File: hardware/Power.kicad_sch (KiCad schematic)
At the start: 33 parts, among them J1 JST XH, J2 JST XH, J22 JST XH, J23 JST XH, J24 JST XH, J25 JST XH, J26 JST XH, J27 JST XH, Q1 NCE40P40K, U4 AMS1117-3.3, U5 DCBuck

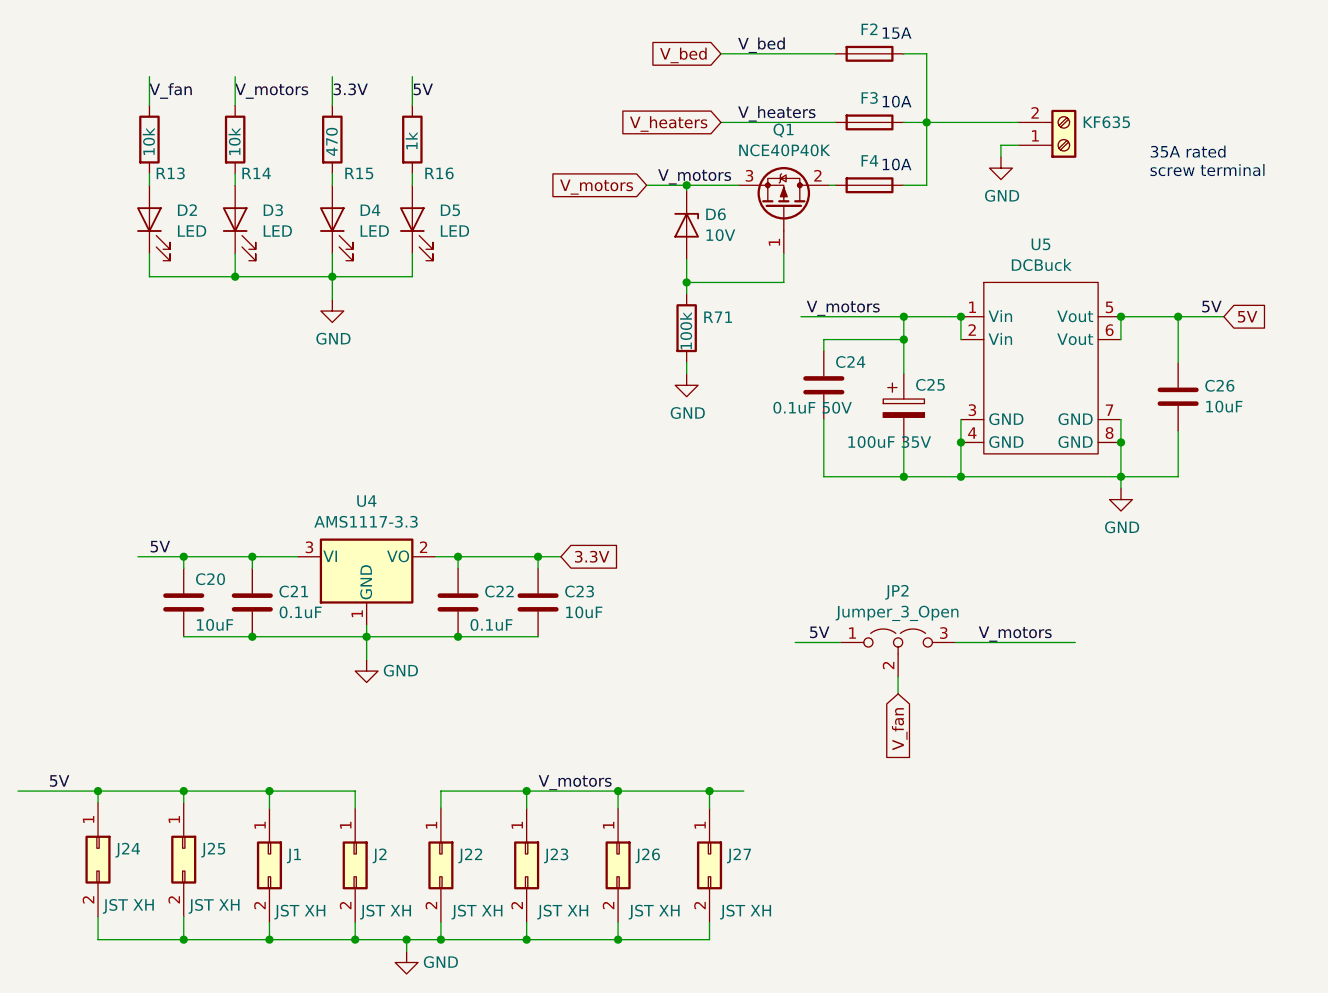
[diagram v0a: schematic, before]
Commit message: Update PrntrBoard fabrication files.
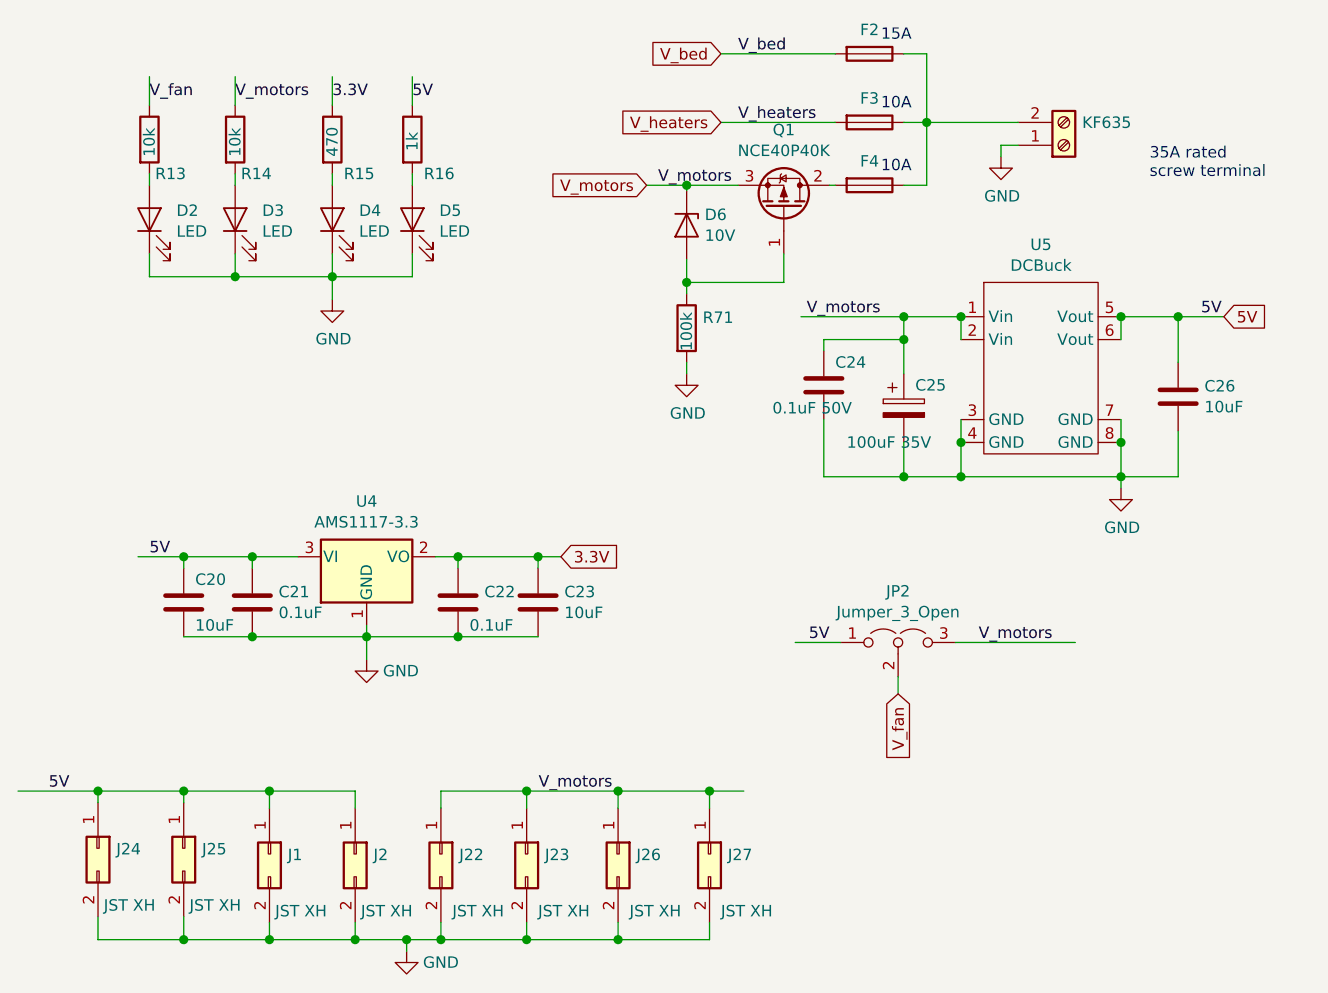
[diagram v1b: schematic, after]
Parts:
- U5: now left out of the parts list
